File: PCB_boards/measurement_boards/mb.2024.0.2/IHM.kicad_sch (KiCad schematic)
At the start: 6 parts

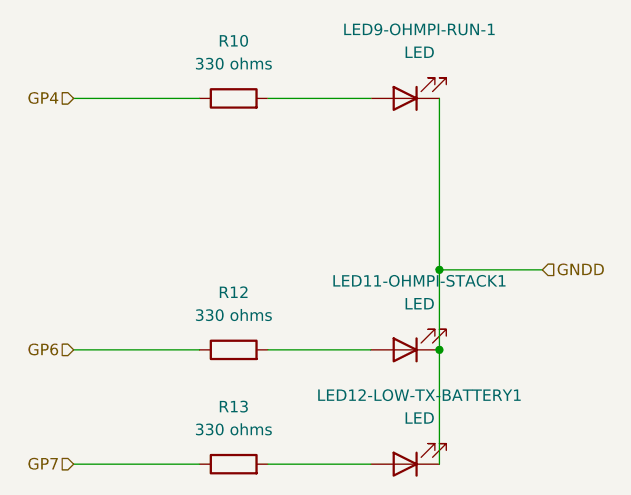
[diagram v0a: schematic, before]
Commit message: update measurement board
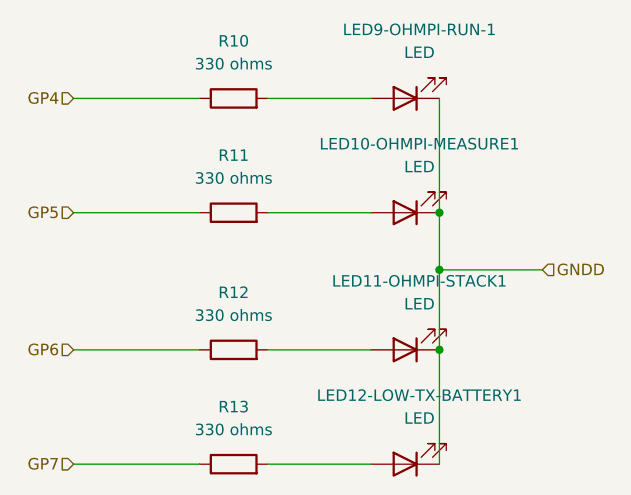
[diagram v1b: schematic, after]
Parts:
- added LED10-OHMPI-MEASURE1: LED, LED_THT:LED_D4.0mm, symbol Device:LED
- added R11: 330 ohms, Resistor_THT:R_Axial_DIN0207_L6.3mm_D2.5mm_P7.62mm_Horizontal, symbol Device:R
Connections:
- net GNDD: now also LED10-OHMPI-MEASURE1.1 (K)
- new net: LED10-OHMPI-MEASURE1.2 (A), R11.2
- new net GP5: R11.1
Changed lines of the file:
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@@
 (kicad_sch (version 20230121) (generator eeschema)
   (paper "A4")
+  (junction (at 152.4 77.47) (diameter 0) (color 0 0 0 0)
+  )
   (junction (at 152.4 92.71) (diameter 0) (color 0 0 0 0)
   )
@@
     (stroke (width 0) (type default))
   )
-  (wire (pts (xy 152.4 64.77) (xy 152.4 83.82))
+  (wire (pts (xy 152.4 77.47) (xy 152.4 83.82))
     (stroke (width 0) (type default))
   )
@@
     (stroke (width 0) (type default))
   )
+  (wire (pts (xy 152.4 64.77) (xy 152.4 77.47))
+    (stroke (width 0) (type default))
+  )
   (wire (pts (xy 111.76 64.77) (xy 125.73 64.77))
     (stroke (width 0) (type default))
   )
+  (wire (pts (xy 111.76 77.47) (xy 125.73 77.47))
+    (stroke (width 0) (type default))
+  )
   (wire (pts (xy 152.4 83.82) (xy 152.4 92.71))
     (stroke (width 0) (type default))
   )
   (wire (pts (xy 152.4 83.82) (xy 163.83 83.82))
+    (stroke (width 0) (type default))
+  )
+  (wire (pts (xy 133.35 77.47) (xy 144.78 77.47))
     (stroke (width 0) (type default))
   )
@@
     (effects (font (size 1.27 1.27)) (justify right))
   )
+  (hierarchical_label "GP5" (shape input) (at 111.76 77.47 180) (fields_autoplaced)
+    (effects (font (size 1.27 1.27)) (justify right))
+  )
   (symbol (lib_id "Device:R") (at 129.54 64.77 90) (unit 1)
     (in_bom yes) (on_board yes) (dnp no) (fields_autoplaced)
@@
         )
       )
+    )
+  )
+  (symbol (lib_id "Device:R") (at 129.54 77.47 90) (unit 1)
+    (in_bom yes) (on_board yes) (dnp no) (fields_autoplaced)
+    (property "Reference" "R11" (at 129.54 71.12 90)
+      (effects (font (size 1.27 1.27)))
+    )
+    (property "Value" "330 ohms" (at 129.54 73.66 90)
+      (effects (font (size 1.27 1.27)))
+    )
+    (property "Footprint" "Resistor_THT:R_Axial_DIN0207_L6.3mm_D2.5mm_P7.62mm_Horizontal" (at 129.54 79.248 90)
+      (effects (font (size 1.27 1.27)) hide)
+    )
+    (property "Datasheet" "~" (at 129.54 77.47 0)
+      (effects (font (size 1.27 1.27)) hide)
+    )
+    (property "Description" "330 ohms resistor" (at 129.54 77.47 90)
+      (effects (font (size 1.27 1.27)) hide)
+    )
+    (pin "1")
+    (pin "2")
+    (instances
+      (project "mb.2024.0.2"
+        (path "/62d2b953-c7cc-4d07-805d-38225011d95a/b5055e4e-7413-40b3-89ed-dfdcecf2a97c"
+          (reference "R11") (unit 1)
+        )
+      )
+    )
+  )
+  (symbol (lib_id "Device:LED") (at 148.59 77.47 180) (unit 1)
+    (in_bom yes) (on_board yes) (dnp no) (fields_autoplaced)
+    (property "Reference" "LED10-OHMPI-MEASURE1" (at 150.1775 69.85 0)
+      (effects (font (size 1.27 1.27)))
+    )
+    (property "Value" "LED" (at 150.1775 72.39 0)
+      (effects (font (size 1.27 1.27)))
+    )
+    (property "Footprint" "LED_THT:LED_D4.0mm" (at 148.59 77.47 0)
+      (effects (font (size 1.27 1.27)) hide)
+    )
+    (property "Datasheet" "~" (at 148.59 77.47 0)
+      (effects (font (size 1.27 1.27)) hide)
+    )
+    (property "Description" "LED" (at 148.59 77.47 0)
+      (effects (font (size 1.27 1.27)) hide)
+    )
+    (pin "1")
+    (pin "2")
+    (instances
+      (project "mb.2024.0.2"
+        (path "/62d2b953-c7cc-4d07-805d-38225011d95a/b5055e4e-7413-40b3-89ed-dfdcecf2a97c"
+          (reference "LED10-OHMPI-MEASURE1") (unit 1)
+        )
+      )
